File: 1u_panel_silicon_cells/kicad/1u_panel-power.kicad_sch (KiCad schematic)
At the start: 66 parts, among them J1 MMS-104-01-[F/L]-SH, Q1 DMP3050LVT-7, Q2 DMP2240UDM-7, U10 TPS63060DSCR, U12 LTC4412, U3 LT1618EMSTRPBF, U4 INA226AIDGSR

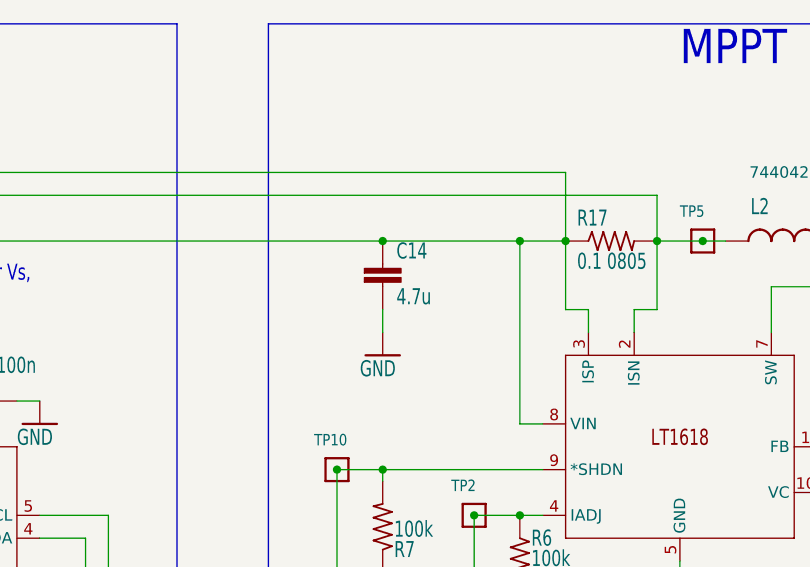
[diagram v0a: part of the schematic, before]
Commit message: updating remote repo for design review
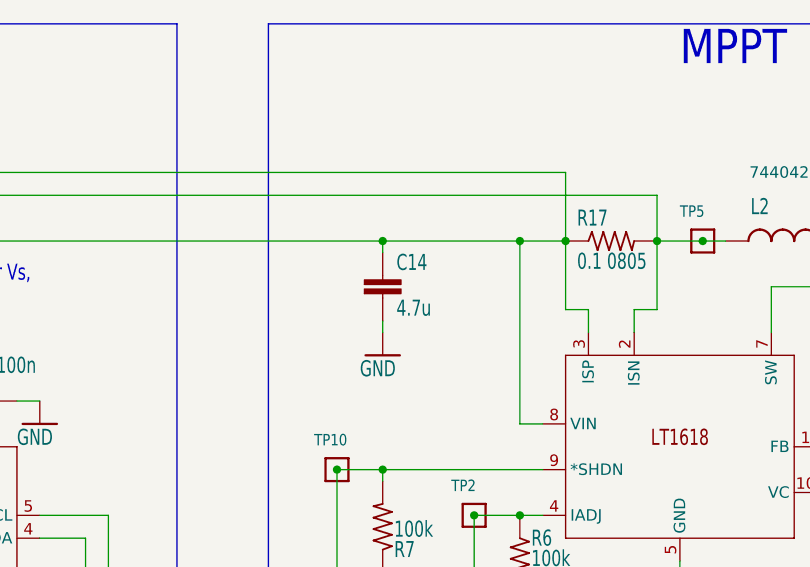
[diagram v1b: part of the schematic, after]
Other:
- moved on the sheet: C14
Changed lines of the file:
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@@
 	(wire
 		(pts
-			(xy 162.56 69.85) (xy 162.56 67.31)
+			(xy 162.56 69.85) (xy 162.56 68.58)
 		)
 		(stroke
@@
 	(wire
 		(pts
+			(xy 162.56 60.96) (xy 162.56 59.69)
+		)
+		(stroke
+			(width 0)
+			(type default)
+		)
+	)
+	(wire
+		(pts
 			(xy 91.44 90.17) (xy 93.98 90.17)
 		)
@@
 	(symbol
 		(lib_id "1u_panel-eagle-import:oresat-rcl_C-EU0603-C-NOSILK")
-		(at 162.56 62.23 0)
+		(at 162.56 63.5 0)
 		(unit 1)
 		(exclude_from_sim no)
@@
 		(dnp no)
 		(property "Reference" "C14"
-			(at 164.084 61.849 0)
+			(at 164.084 63.119 0)
 			(effects
 				(font
@@
 		)
 		(property "Value" "4.7u"
-			(at 164.084 66.929 0)
+			(at 164.084 68.199 0)
 			(effects
 				(font
@@
 		)
 		(property "Footprint" "1u_panel:.0603-C-NOSILK"
-			(at 162.56 62.23 0)
+			(at 162.56 63.5 0)
 			(effects
 				(font
@@
 		)
 		(property "Datasheet" ""
-			(at 162.56 62.23 0)
+			(at 162.56 63.5 0)
 			(effects
 				(font
@@
 		)
 		(property "Description" ""
-			(at 162.56 62.23 0)
+			(at 162.56 63.5 0)
 			(effects
 				(font
@@
 		)
 		(property "DIS" "Digi-Key"
-			(at 162.56 62.23 0)
+			(at 162.56 63.5 0)
 			(effects
 				(font
@@
 		)
 		(property "DPN" "587-4332-1-ND"
-			(at 162.56 62.23 0)
+			(at 162.56 63.5 0)
 			(effects
 				(font
@@
 		)
 		(property "MFR" "Taiyo"
-			(at 162.56 62.23 0)
+			(at 162.56 63.5 0)
 			(effects
 				(font
@@
 		)
 		(property "MPN" "EMK107BBJ475KAHT"
-			(at 162.56 62.23 0)
+			(at 162.56 63.5 0)
 			(effects
 				(font
